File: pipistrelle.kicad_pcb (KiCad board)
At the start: 2 copper layers, 211.2 x 85.2 mm, 30 parts, among them SW10 SW_Push, SW11 SW_Push, SW12 SW_Push, SW14 SW_Push, SW15 SW_Push, SW16 SW_Push, SW17 SW_Push, SW18 SW_Push, SW2 SW_Push, SW20 SW_Push, SW21 SW_Push, SW22 SW_Push, SW23 SW_Push, SW24 SW_Push, SW25 SW_Push, SW26 SW_Push, SW3 SW_Push, SW4 SW_Push, SW5 SW_Push, SW6 SW_Push, SW8 SW_Push, SW9 SW_Push, U1 ProMicro-kbd

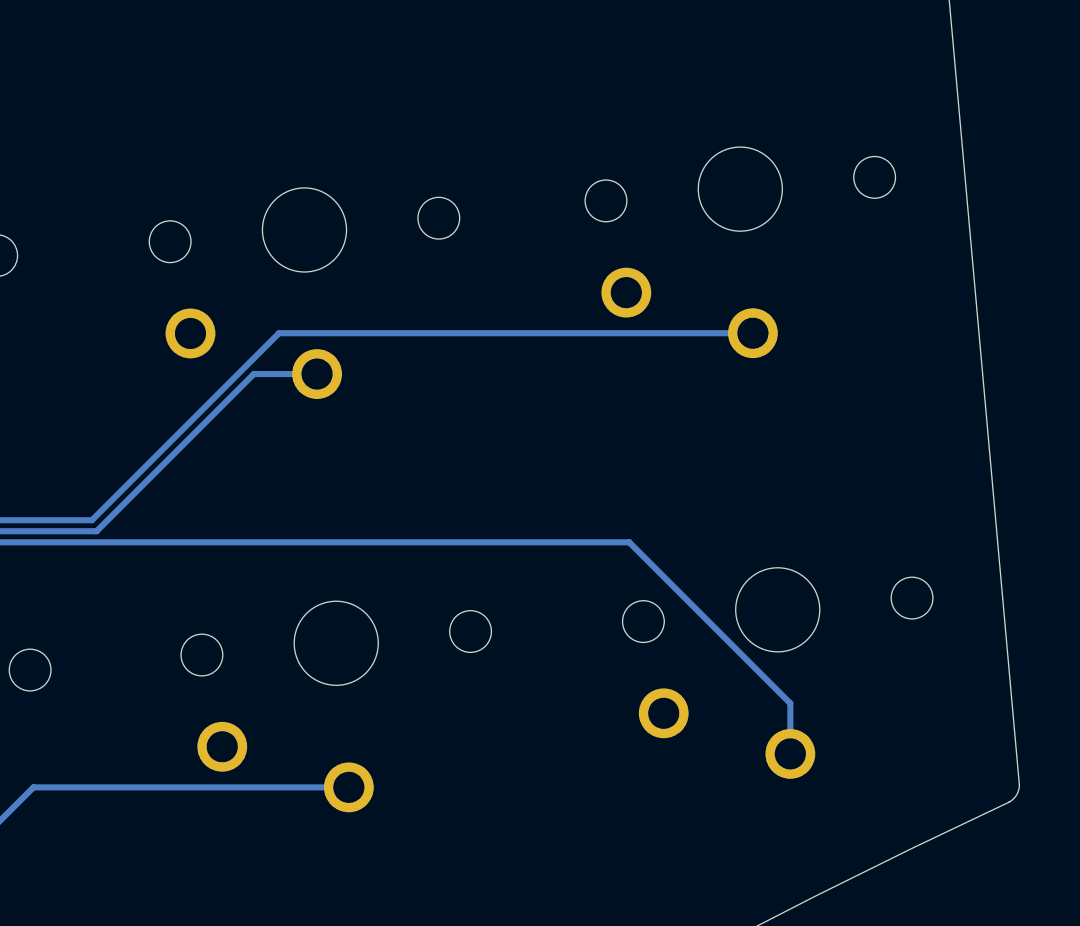
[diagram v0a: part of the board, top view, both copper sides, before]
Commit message: Add files via upload
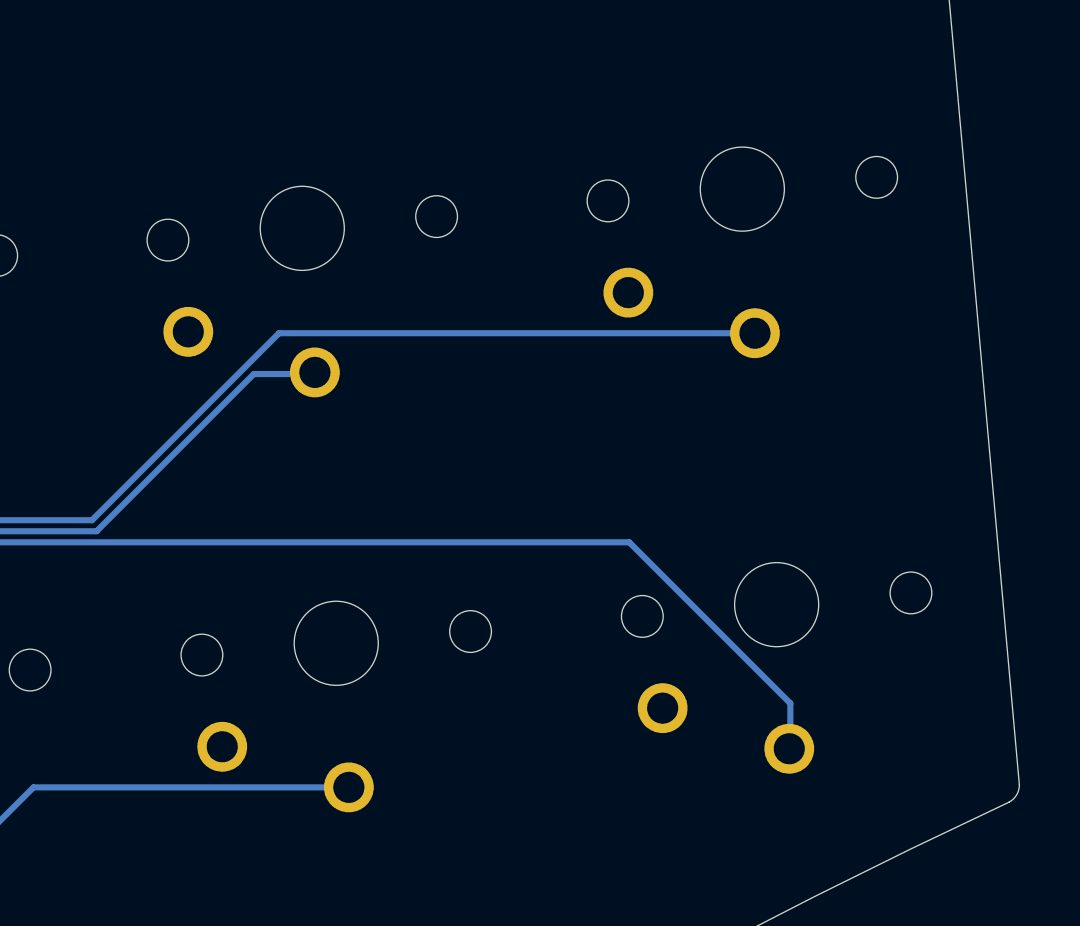
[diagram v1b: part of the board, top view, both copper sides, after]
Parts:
- moved SW2 0.21 mm to (225.0, 98.8)
- moved SW17 0.11 mm to (205.7, 83.5)
- moved SW12 0.08 mm to (223.6, 81.9)

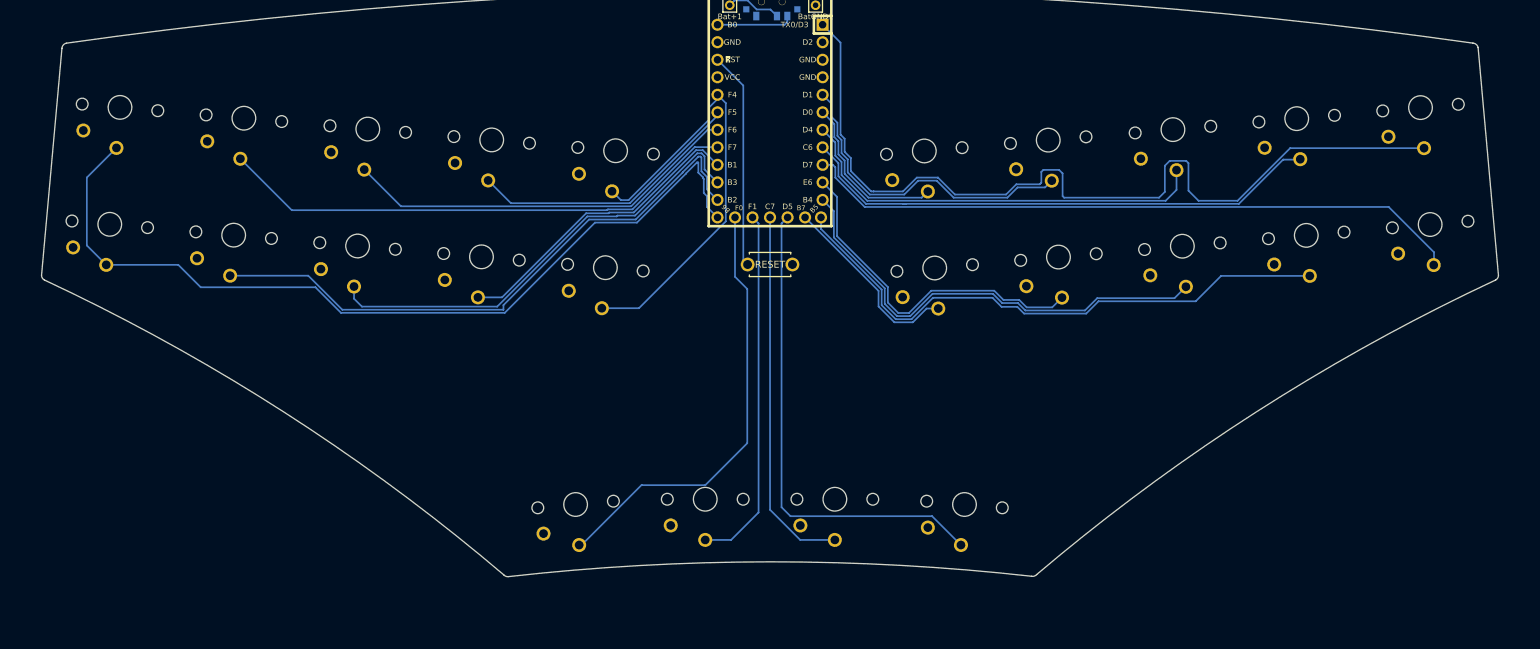
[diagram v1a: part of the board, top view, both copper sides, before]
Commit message: Add files via upload
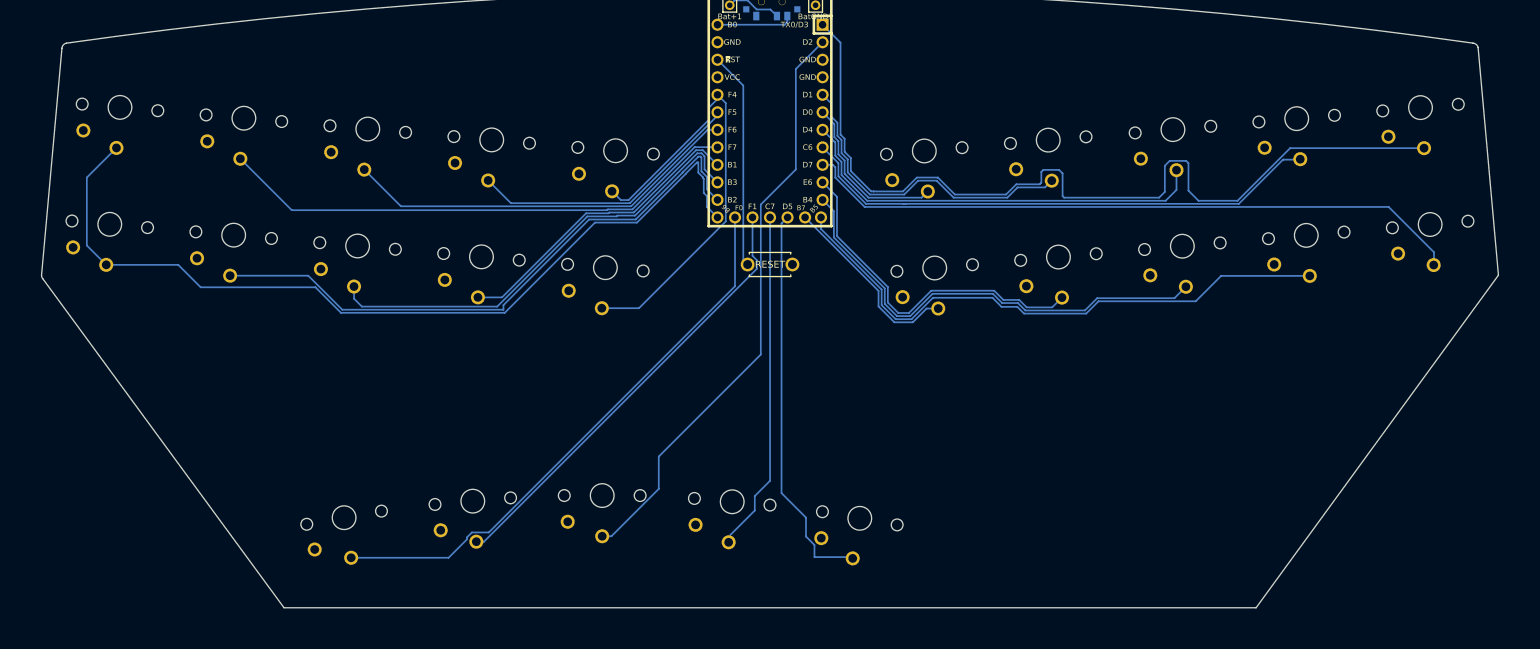
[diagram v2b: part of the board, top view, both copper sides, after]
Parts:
- added SW18: SW_Push, Kailh:SW_PG1350_nonrev_DPB2, F.Cu at (105.0, 138.2)
- moved SW25 33.7 mm to (86.2, 139.0), turned to 5 degrees
- moved SW26 33.6 mm to (67.5, 141.4), turned to 10 degrees
- moved SW23 15.3 mm to (142.3, 141.4), turned to 350 degrees
- moved SW24 14.9 mm to (123.8, 139.1), turned to 355 degrees
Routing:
- net Switch18: track 0.00 -> 85.6 mm
- net Switch23: track 64.0 -> 82.1 mm
- net Switch20: track 70.7 -> 57.2 mm
- net Switch22: track 52.5 -> 64.8 mm
- net Switch21: track 53.6 -> 50.4 mm
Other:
- board size 211.2 x 85.2 mm -> 211.2 x 89.7 mm
